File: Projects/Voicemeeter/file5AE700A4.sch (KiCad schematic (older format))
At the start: 18 parts, among them J501 CONN_01X05, J502 CONN_01X03, J503 CONN_01X05, J504 CONN_01X02, J505 CONN_01X03, J506 CONN_01X02, J507 DIN_5, J508 DIN_5, J509 Screw_Terminal_1x02, SW501 SW_Push, U501 stm32f103-china-MS, U502 PC817

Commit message: fixed a header
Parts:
- removed J501: CONN_01X05, Pin_Headers:Pin_Header_Straight_1x05_Pitch2.54mm, symbol CONN_01X05
- removed J502: CONN_01X03, Pin_Headers:Pin_Header_Straight_1x03_Pitch2.54mm, symbol CONN_01X03
- added J501: Conn_01x08, Pin_Headers:Pin_Header_Straight_1x08_Pitch2.54mm, symbol Conn_01x08
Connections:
- wire segments 80 -> 91

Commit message: gtg
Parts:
- removed J501: Conn_01x08, Pin_Headers:Pin_Header_Straight_1x08_Pitch2.54mm, symbol Conn_01x08
- removed J503: CONN_01X05, Pin_Headers:Pin_Header_Straight_1x05_Pitch2.54mm, symbol CONN_01X05
- removed J504: CONN_01X02, Pin_Headers:Pin_Header_Straight_1x02_Pitch2.54mm, symbol CONN_01X02
- added J?: SPARE, symbol Conn_01x05
- added R? (x3): R, symbol R
- added SW?: Rotary_Encoder_Switch, symbol Rotary_Encoder_Switch
- J505: value CONN_01X03 -> MIDI OUT
- J506: value CONN_01X02 -> MIDI IN
- renumbered SW501 to RESET1
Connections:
- net labels added: OLED1, OLED2, OLED3, OLED4, OLED5, OLED6, OLED7, OLED[1..7], ROT1, ROT2, ROT3
- wire segments 91 -> 110

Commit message: taking a break
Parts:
- removed J507, J508: DIN_5, symbol DIN_5
- removed J509: Screw_Terminal_1x02, TerminalBlock:TerminalBlock_bornier-2_P5.08mm, symbol Screw_Terminal_1x02
- added J2: Screw_Terminal_01x02, symbol Screw_Terminal_01x02
- added J3, J4: DIN-5_180degree, symbol DIN-5_180degree
- added OLED1: 1.5\"OLED, symbol 1.5"OLED
- J505: symbol CONN_01X03 -> Conn_01x03
- J506: symbol CONN_01X02 -> Conn_01x02
- R1, R2, R3: renamed from R?; value R -> 10k
- gave numbers to parts that had none: 2
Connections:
- net labels removed: OLED[1..7]
- wire segments 110 -> 98
- no-connect marks 14 -> 16
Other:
- moved on the sheet: R503

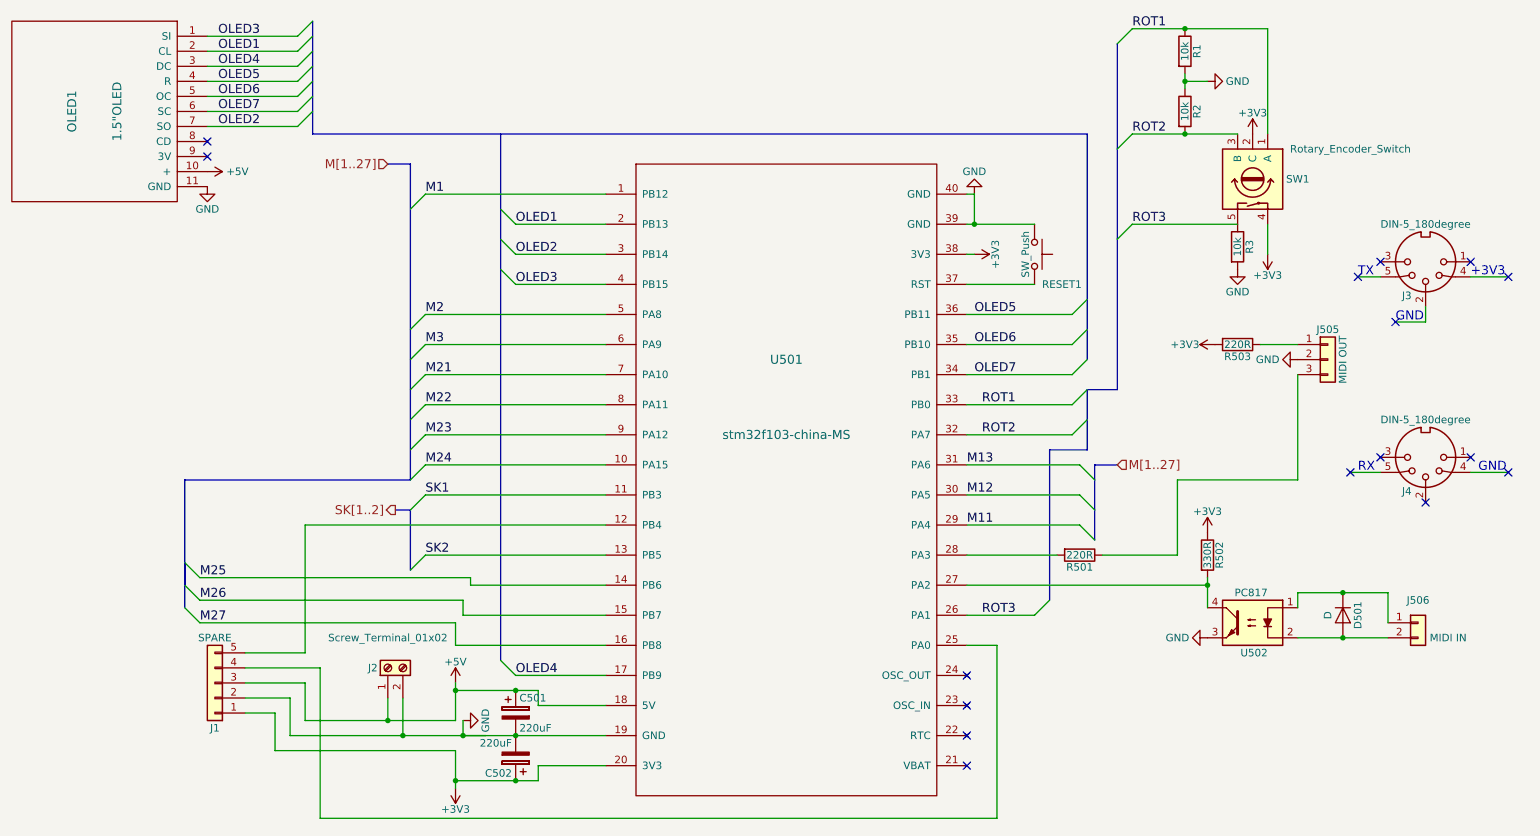
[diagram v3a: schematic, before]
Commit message: stuff
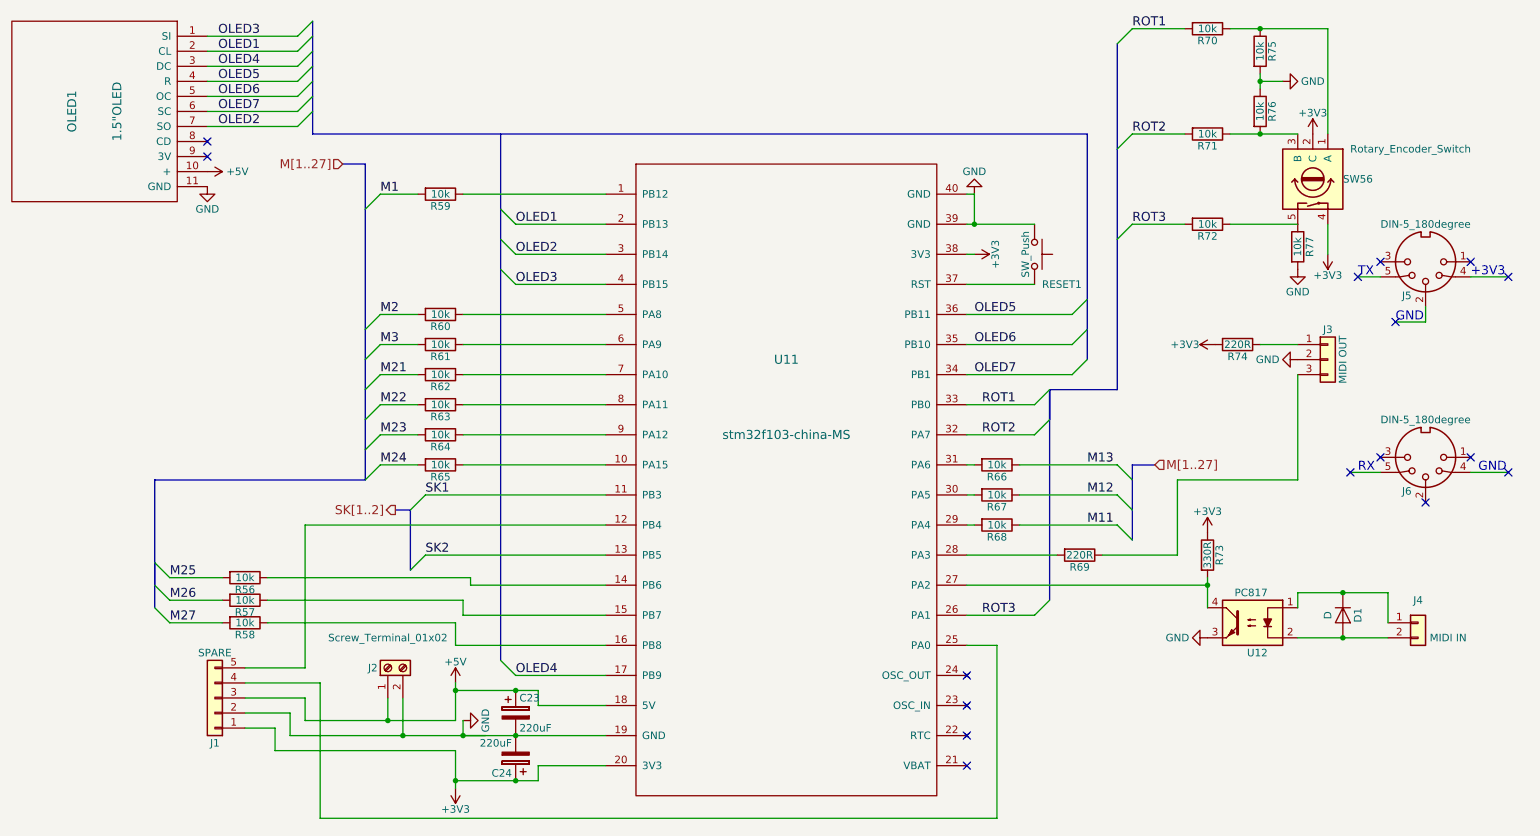
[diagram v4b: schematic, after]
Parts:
- added R56, R57, R58, R59, R60, R61, R62, R63, R64, R65, R66, R67, R68, R70, R71, R72: 10k, symbol R
- renumbered C501 to C23, C502 to C24, D501 to D1, J505 to J3, J506 to J4, J3 to J5, J4 to J6, R501 to R69, R502 to R73, R503 to R74, R1 to R75, R2 to R76, R3 to R77, SW1 to SW56, U501 to U11, U502 to U12
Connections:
- net M1: now also R59.2; no longer U11.1 (PB12)
- net M11: now also R68.1; no longer U11.29 (PA4)
- net M12: now also R67.1; no longer U11.30 (PA5)
- net M13: now also R66.1; no longer U11.31 (PA6)
- net M2: now also R60.2; no longer U11.5 (PA8)
- net M21: now also R62.2; no longer U11.7 (PA10)
- net M22: now also R63.2; no longer U11.8 (PA11)
- net M23: now also R64.2; no longer U11.9 (PA12)
- net M24: now also R65.2; no longer U11.10 (PA15)
- net M25: now also R56.2; no longer U11.14 (PB6)
- net M26: now also R57.2; no longer U11.15 (PB7)
- net M27: now also R58.2; no longer U11.16 (PB8)
- net M3: now also R61.2; no longer U11.6 (PA9)
- net ROT1: now also R70.2; no longer R75.1, SW56.1 (A)
- net ROT2: now also R71.2; no longer R76.2, SW56.3 (B)
- net ROT3: now also R72.2; no longer R77.1, SW56.5
- new net: R59.1, U11.1 (PB12)
- new net: R65.1, U11.10 (PA15)
- new net: R56.1, U11.14 (PB6)
- new net: R57.1, U11.15 (PB7)
- new net: R58.1, U11.16 (PB8)
- new net: R68.2, U11.29 (PA4)
- new net: R67.2, U11.30 (PA5)
- new net: R66.2, U11.31 (PA6)
- new net: R60.1, U11.5 (PA8)
- new net: R61.1, U11.6 (PA9)
- new net: R62.1, U11.7 (PA10)
- new net: R63.1, U11.8 (PA11)
- new net: R64.1, U11.9 (PA12)
- new net: R70.1, R75.1, SW56.1 (A)
- new net: R71.1, R76.2, SW56.3 (B)
- new net: R72.1, R77.1, SW56.5
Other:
- moved on the sheet: J1, R75, R76, R77, SW56

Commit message: stuff
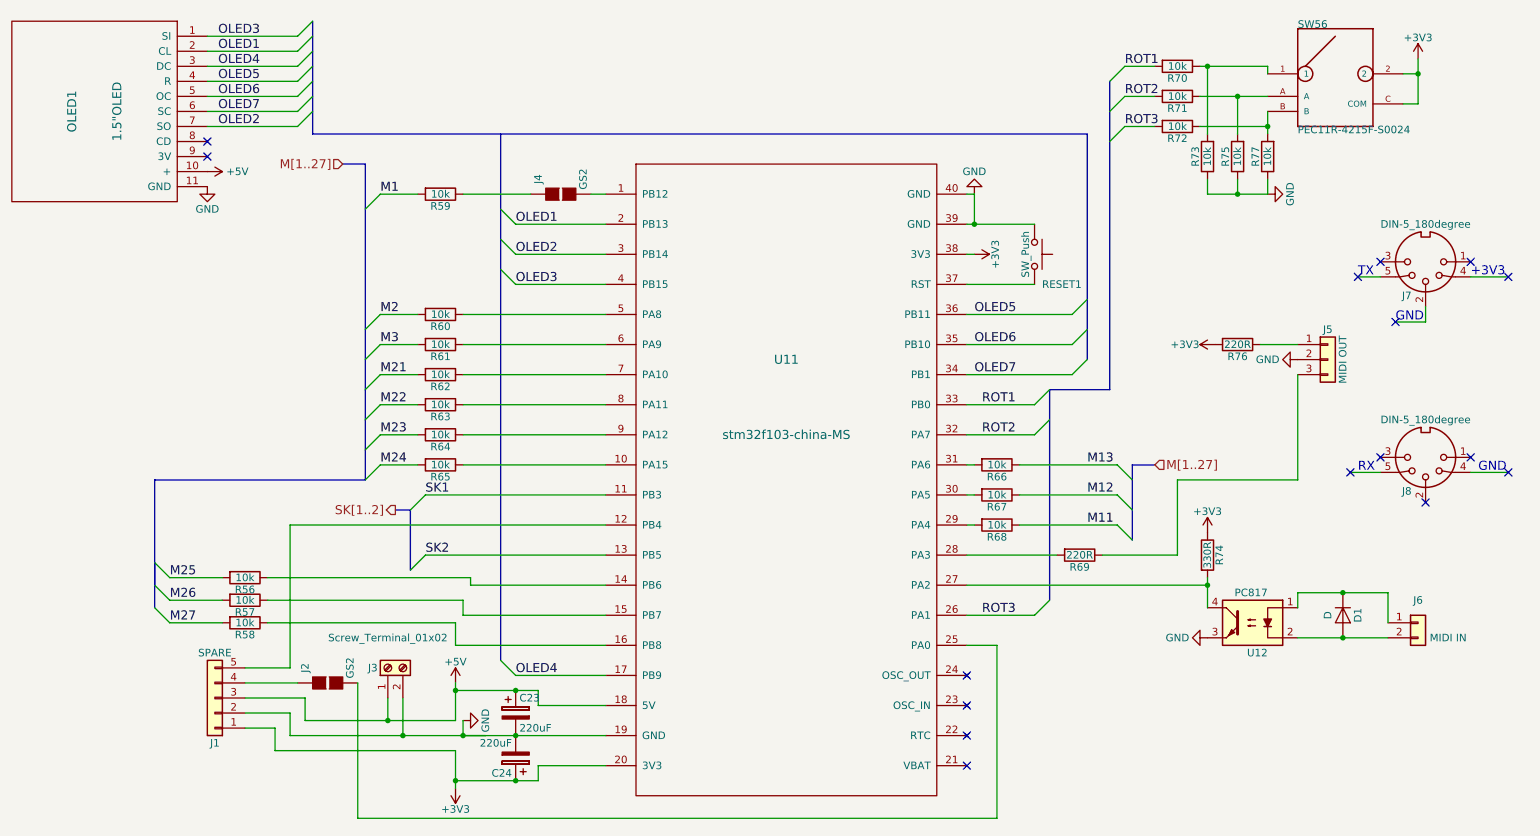
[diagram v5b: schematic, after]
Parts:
- removed R76: 10k, symbol R
- removed SW56: Rotary_Encoder_Switch, symbol Rotary_Encoder_Switch
- added J2, J4: GS2, MATHSTERK:SB2, symbol GS2
- added R73: 10k, Resistors_SMD:R_1206_HandSoldering, symbol R
- added SW56: PEC11R-4215F-S0024, MATHSTERK:Rotary_Encoder_Switched_PEC11R, symbol PEC11R-4215F-S0024
- J1: footprint (none) -> Pin_Headers:Pin_Header_Straight_1x05_Pitch2.54mm
- J3: renamed from J2; footprint (none) -> Connectors_Terminal_Blocks:TerminalBlock_Altech_AK300-2_P5.00mm
- R56, R57, R58, R59, R60, R61, R62, R63, R64, R65, R66, R67, R68, R70, R71, R72, R75, R77: footprint (none) -> Resistors_SMD:R_1206_HandSoldering
- U11: footprint myelin-kicad:stm32f103c8t6-module-china-MS -> (none)
- renumbered J3 to J5, J4 to J6, J5 to J7, J6 to J8, R73 to R74, R74 to R76
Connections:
- net +3V3: now also SW56.2, SW56.C (COM)
- net GND: now also R75.1, R77.1, R73.1; no longer R75.2, R77.2
- net at R59.1: now also J4.1 (G1); no longer U11.1 (PB12)
- net at J1.4 (Pin_4): now also J2.1 (G1); no longer U11.25 (PA0)
- net at R70.1: now also R73.2, SW56.1; no longer R75.1
- net at R71.1: now also R75.2, SW56.A
- net at R72.1: now also R77.2, SW56.B; no longer R77.1
- new net: J2.2 (G2), U11.25 (PA0)
- new net: J4.2 (G2), U11.1 (PB12)
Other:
- moved on the sheet: R70, R71, R72
